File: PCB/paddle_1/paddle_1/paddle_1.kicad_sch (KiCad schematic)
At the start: 1 part, among them J1 Conn_01x02_Pin

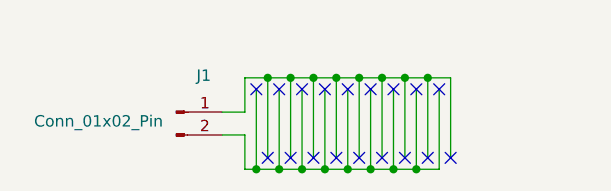
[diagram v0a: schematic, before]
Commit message: created repo
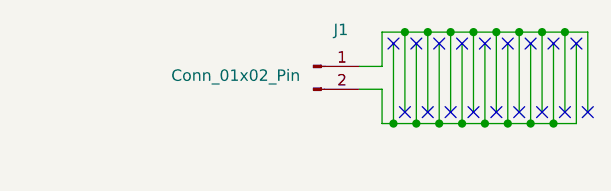
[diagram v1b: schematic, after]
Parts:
- J1: footprint (none) -> Connector_PinHeader_2.54mm:PinHeader_2x01_P2.54mm_Vertical
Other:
- moved on the sheet: J1
